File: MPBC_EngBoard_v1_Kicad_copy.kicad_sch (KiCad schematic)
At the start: 19 parts, among them Q1 BSZ018N04LS6, Q2 BSZ018N04LS6, U1 LM1084-ADJ, U2 MP1909

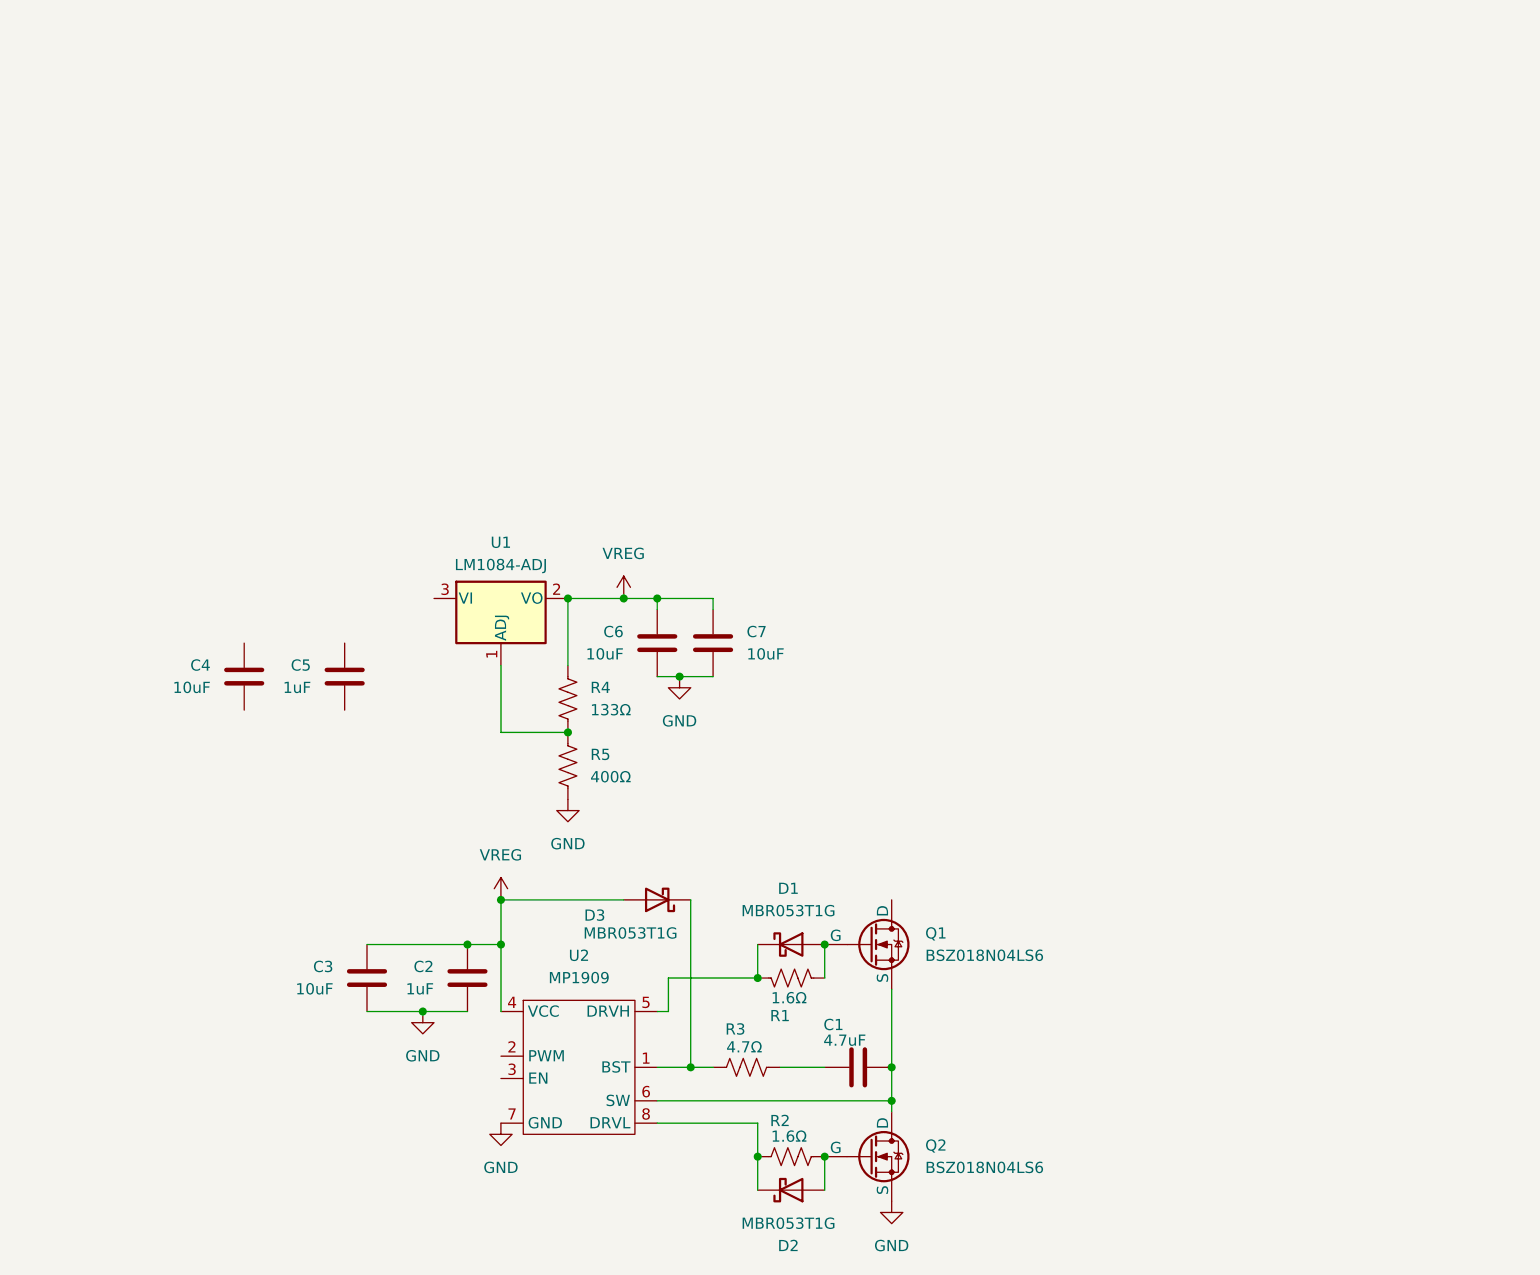
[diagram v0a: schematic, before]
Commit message: Buck Converter Circuit Finished
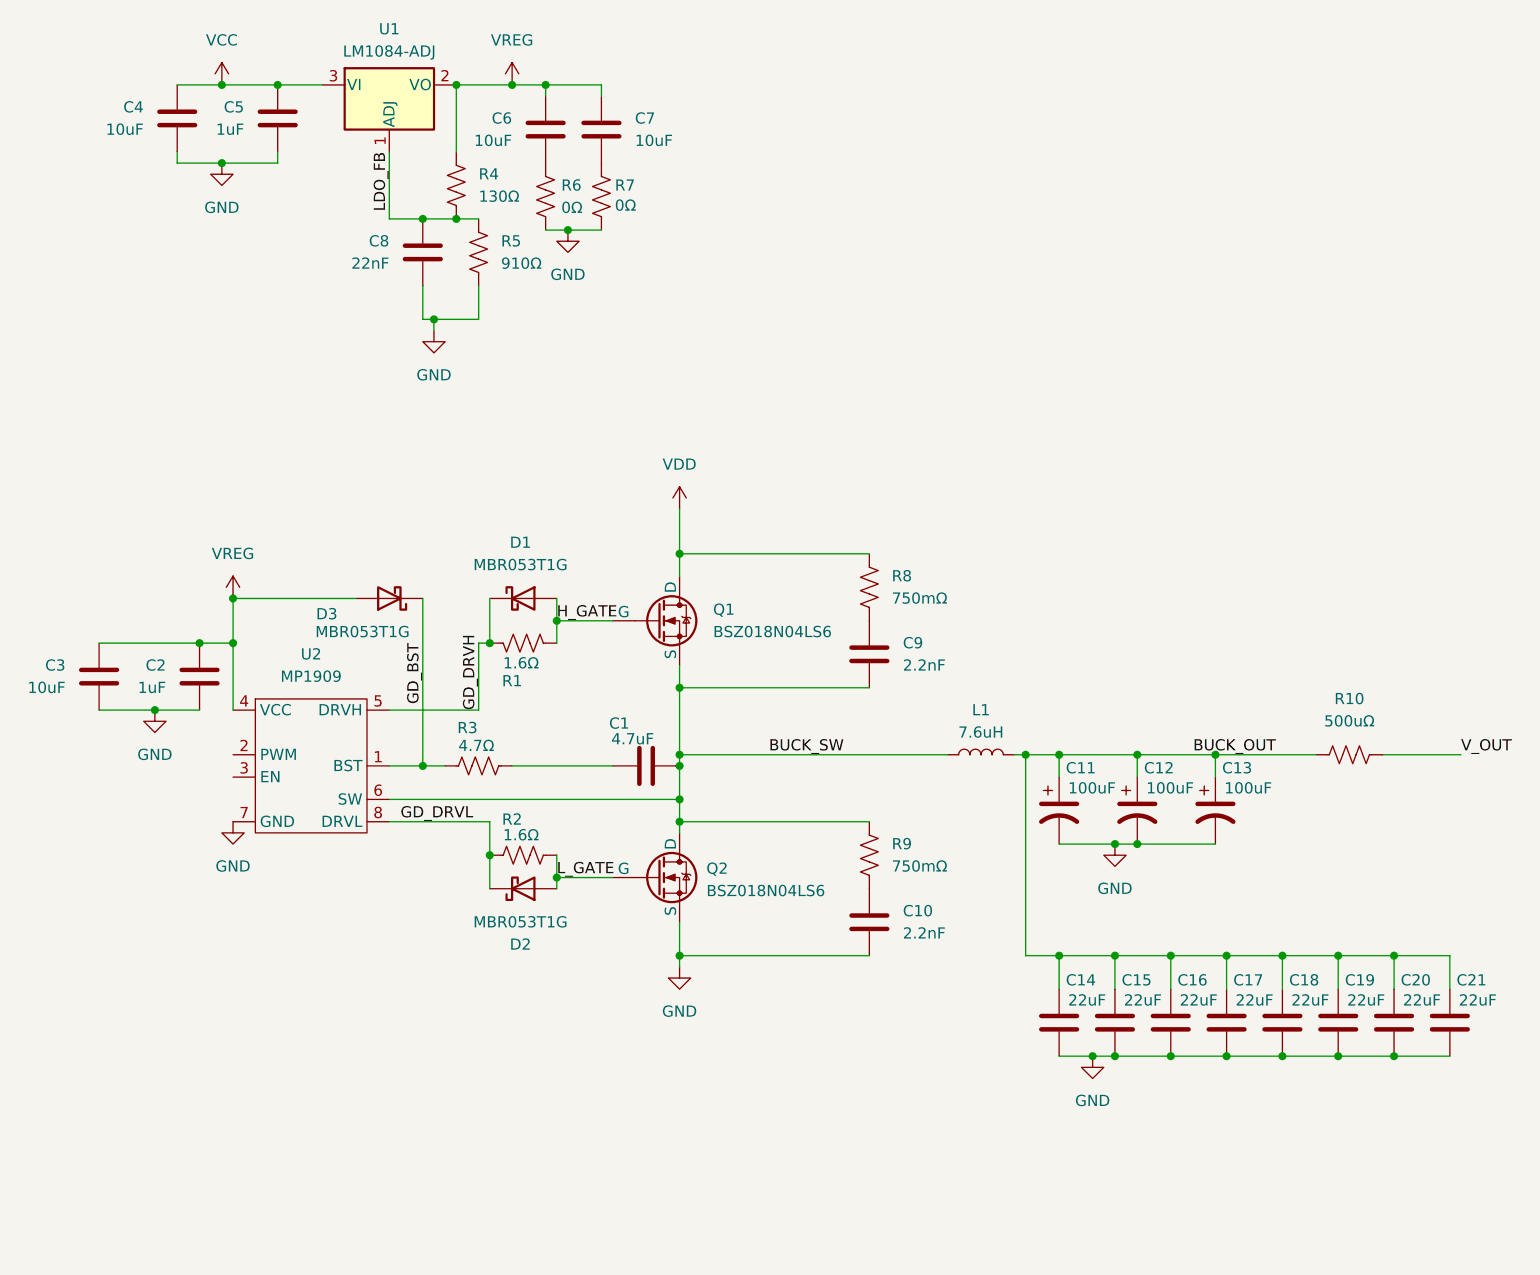
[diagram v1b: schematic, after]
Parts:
- added C10, C9: 2.2nF, symbol Device:C
- added C11, C12, C13: 100uF, symbol Device:C_Polarized_US
- added C14, C15, C16, C17, C18, C19, C20, C21: 22uF, symbol Device:C
- added C8: 22nF, 0603, symbol Device:C
- added L1: 7.6uH, symbol Device:L
- added R10: 500uΩ, symbol Device:R_US
- added R6, R7: 0Ω, symbol Device:R_US
- added R8, R9: 750mΩ, symbol Device:R_US
- R4: value 133Ω -> 130Ω
- R5: value 400Ω -> 910Ω
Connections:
- net GND: now also C4.2, C5.2, C10.2, C11.2, C12.2, C13.2, C14.2, C15.2, C16.2, C17.2, C18.2, C19.2, C20.2, C21.2, C8.2, R6.2, R7.2; no longer C6.2, C7.2
- net BUCK_SW: now reaches C1.2, Q1.3 (S), Q2.1 (D), U2.6 (SW)
- net BUCK_SW: now also C9.2, L1.1, R9.1
- net VCC: now reaches C5.1
- net VCC: now also C4.1, U1.3 (VI)
- net VDD: now reaches Q1.1 (D)
- net VDD: now also R8.1
- net H_GATE: now reaches D1.2 (A), Q1.2 (G), R1.1
- net LDO_FB: now reaches R4.2, R5.1, U1.1 (ADJ)
- net LDO_FB: now also C8.1
- net GD_DRVH: now reaches D1.1 (K), R1.2, U2.5 (DRVH)
- net GD_DRVL: now reaches D2.1 (K), R2.2, U2.8 (DRVL)
- net L_GATE: now reaches D2.2 (A), Q2.2 (G), R2.1
- net GD_BST: now reaches D3.1 (K), R3.2, U2.1 (BST)
- new net: C9.1, R8.2
- new net: C10.1, R9.2
- new net: C6.2, R6.1
- new net: C7.2, R7.1
- new net BUCK_OUT: C11.1, C12.1, C13.1, C14.1, C15.1, C16.1, C17.1, C18.1, C19.1, C20.1, C21.1, L1.2, R10.1
- new net V_OUT: R10.2
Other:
- moved on the sheet: C1, C2, C3, C4, C5, C6, C7, D1, D2, D3, Q1, Q2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
